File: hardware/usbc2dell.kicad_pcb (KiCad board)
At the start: 2 copper layers, 39.5 x 26.5 mm, 27 parts, among them J1 TYPE-C-31-M-17, J2 DELL_Charger, Q1 MDD50N03D, Q2 MMBT5551, SW1 SW_DIP_x04, U1 ATtiny1616-M, U2 FUSB302BMPX, U3 L7805, U4 SRV05-4

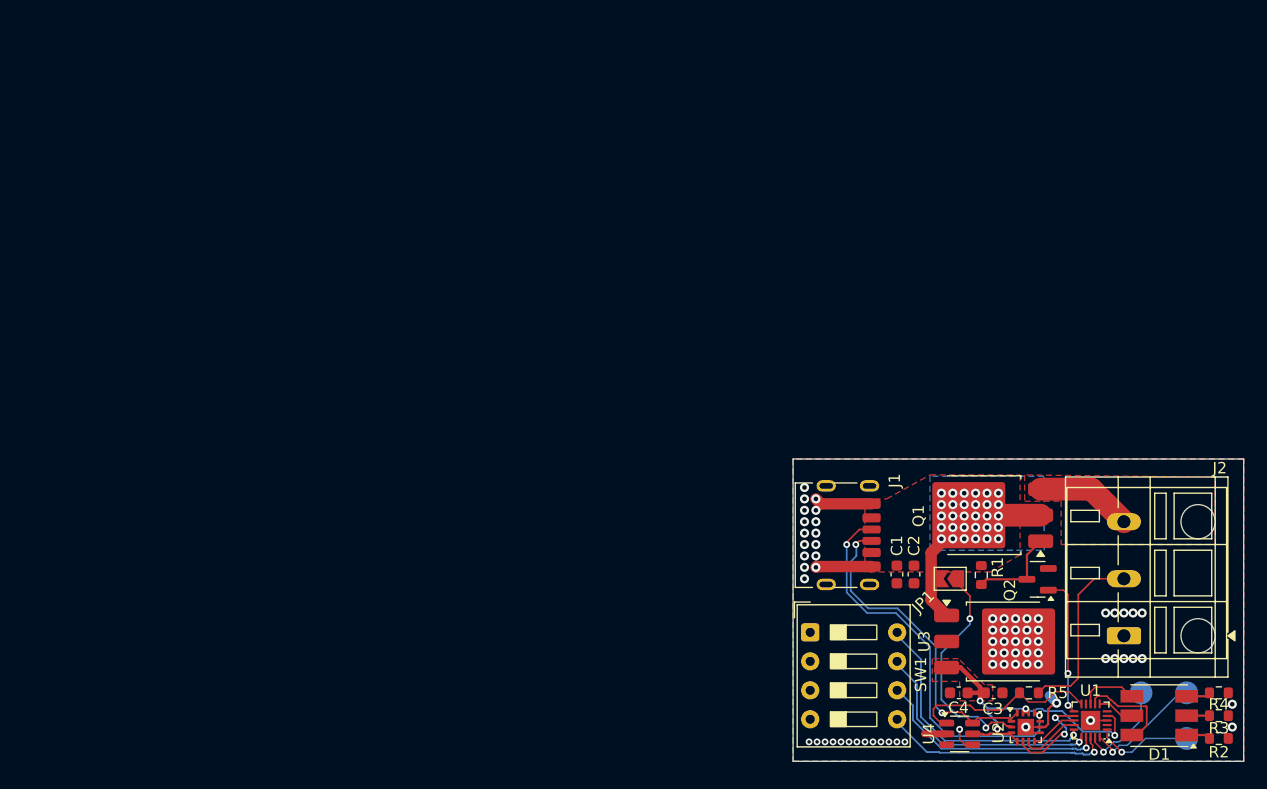
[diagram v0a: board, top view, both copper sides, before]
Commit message: move PCB
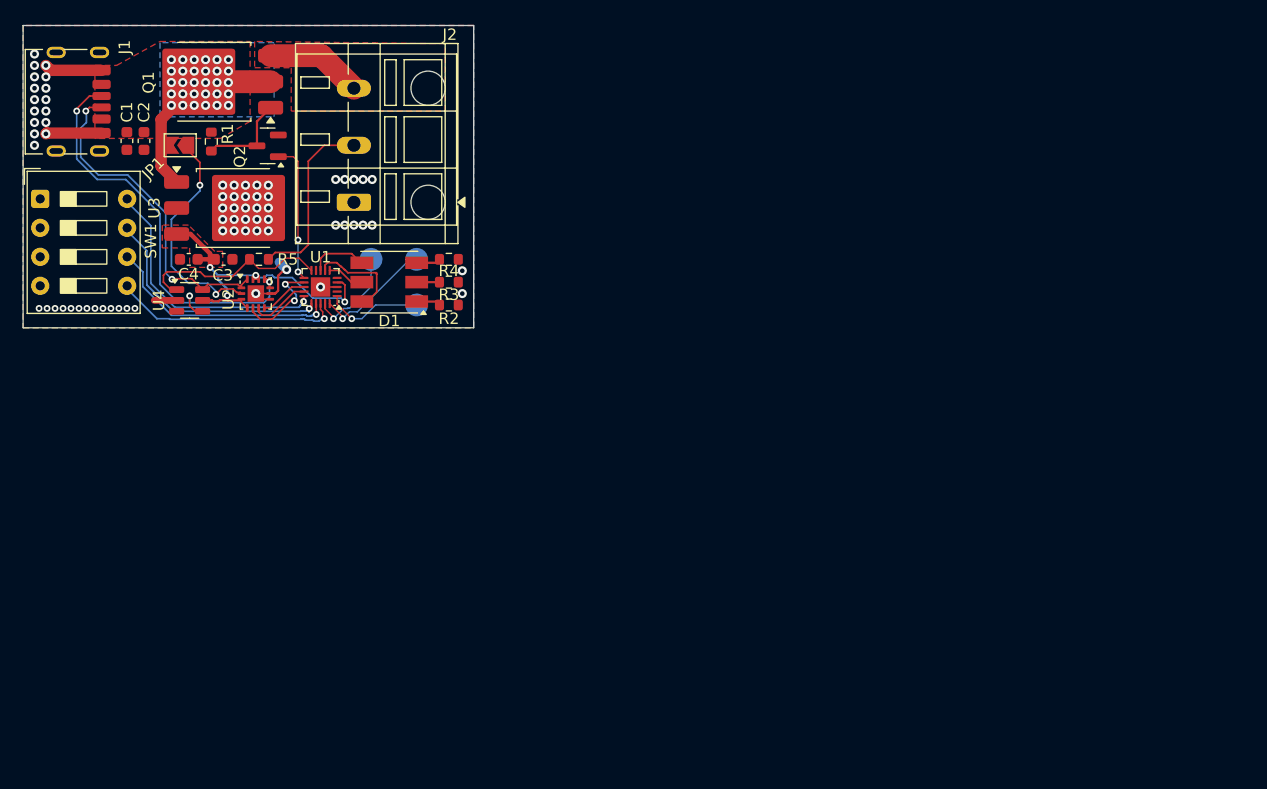
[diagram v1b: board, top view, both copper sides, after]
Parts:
- moved J1 77.5 mm to (23.7, 26.7)
- moved C1 77.5 mm to (29.1, 30.1)
- moved C2 77.5 mm to (30.6, 30.1)
- moved C3 77.5 mm to (37.6, 40.5)
- moved C4 77.5 mm to (34.5, 40.5)
- moved D1 77.5 mm to (52.1, 42.5)
- moved J2 77.5 mm to (49.0, 35.5)
- moved JP1 77.5 mm to (33.8, 30.5)
- moved Q1 77.5 mm to (36.7, 24.9)
- moved Q2 77.5 mm to (41.4, 30.6)
- moved R1 77.5 mm to (36.5, 30.2)
- moved R2 77.5 mm to (57.3, 44.5)
- moved R3 77.5 mm to (57.3, 42.5)
- moved R4 77.5 mm to (57.3, 40.5)
- moved R5 77.5 mm to (40.7, 40.5)
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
